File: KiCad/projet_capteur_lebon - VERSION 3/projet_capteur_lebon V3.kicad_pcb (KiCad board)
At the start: 2 copper layers, 85.2 x 66 mm, 25 parts, among them J1 Power, J2 Digital/PWM, J3 Analog, J4 Digital/PWM

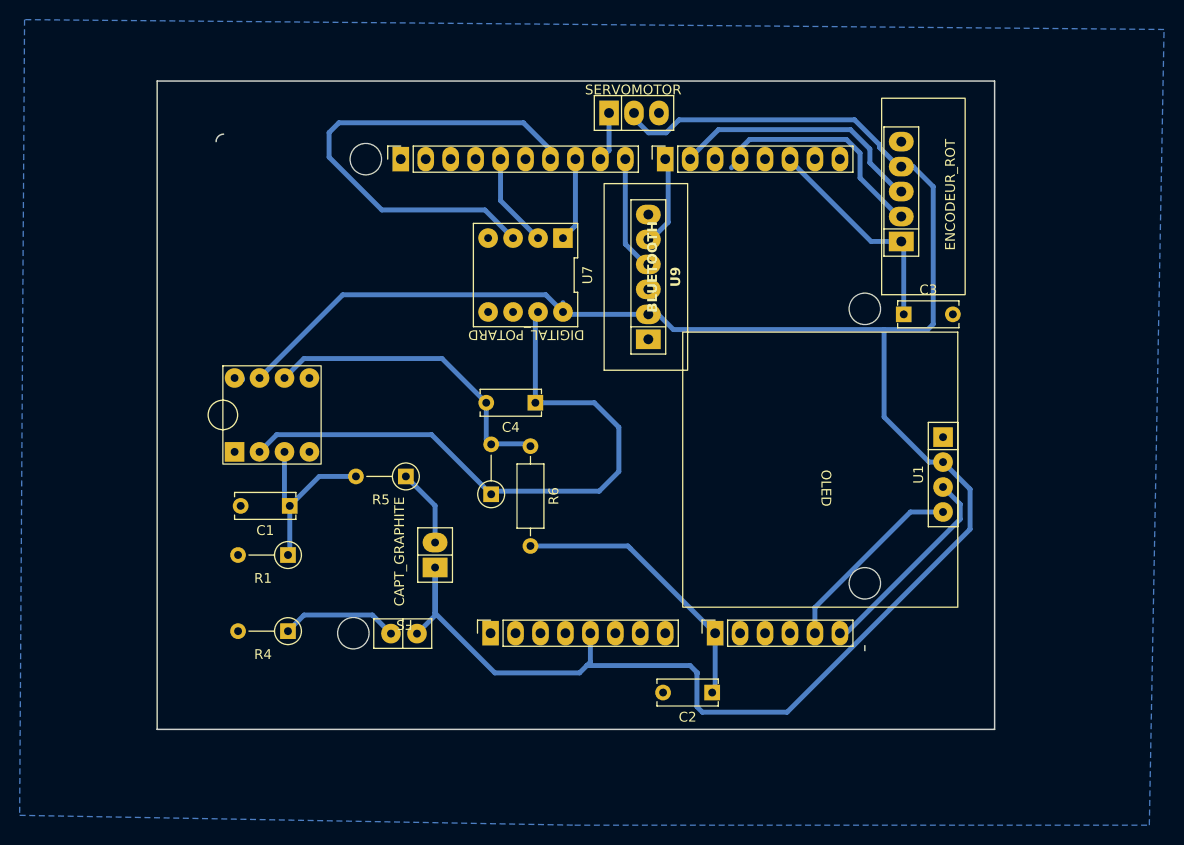
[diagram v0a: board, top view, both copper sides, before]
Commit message: version finale validee par cathy qui sera imprimee
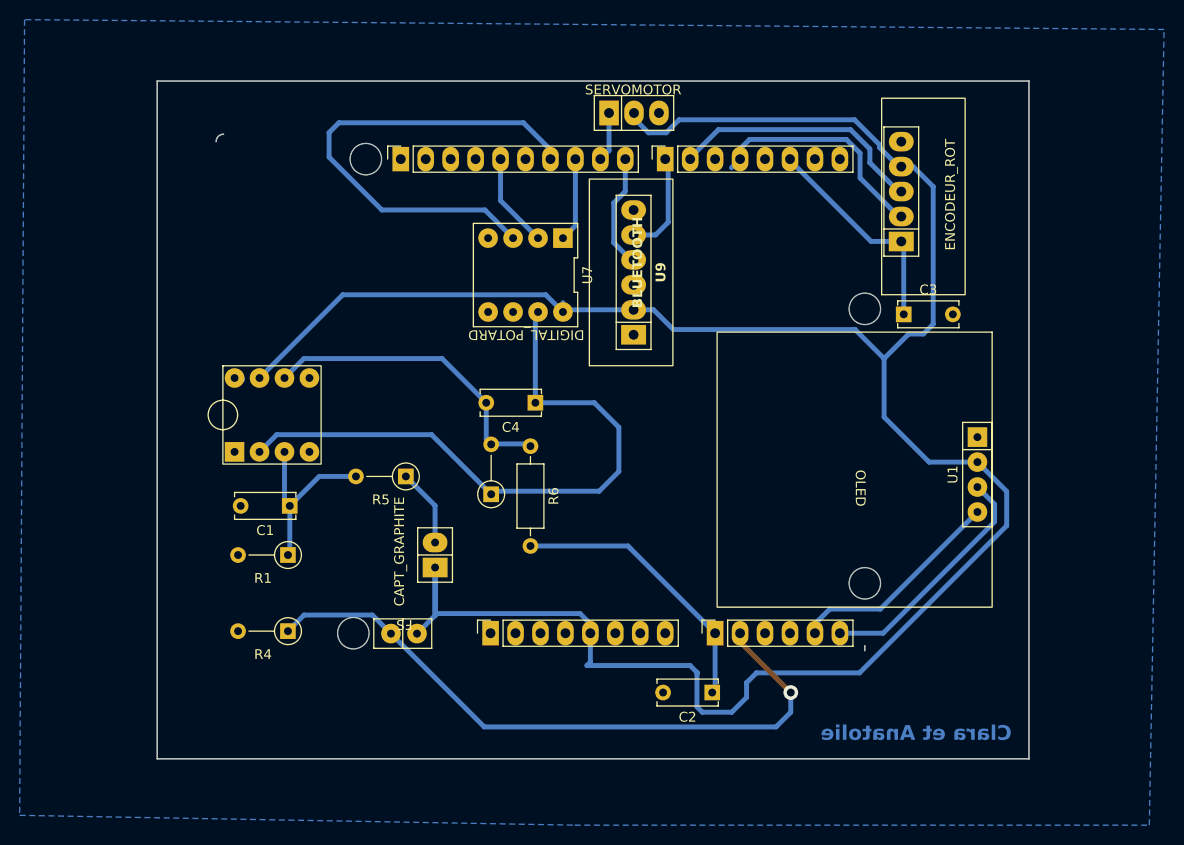
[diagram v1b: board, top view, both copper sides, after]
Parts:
- moved U1 3.50 mm to (177.5, 81.3)
- moved U9 1.57 mm to (142.5, 60.7)
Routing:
- net OUT_FLEX: track 12.6 -> 68.0 mm, vias 0 -> 1
- net 5V: track 233.3 -> 240.7 mm
- net SCL: track 21.4 -> 25.1 mm
- net SDA: track 19.7 -> 22.2 mm
- net RX: track 9.30 -> 10.5 mm
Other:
- board size 85.2 x 66 mm -> 88.8 x 69 mm
- board text added: "Clara et Anatolie"
